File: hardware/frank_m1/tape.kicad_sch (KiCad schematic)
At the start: 11 parts, among them J11 SJ1-353XNG, Q1 BC850, Q2 BC850

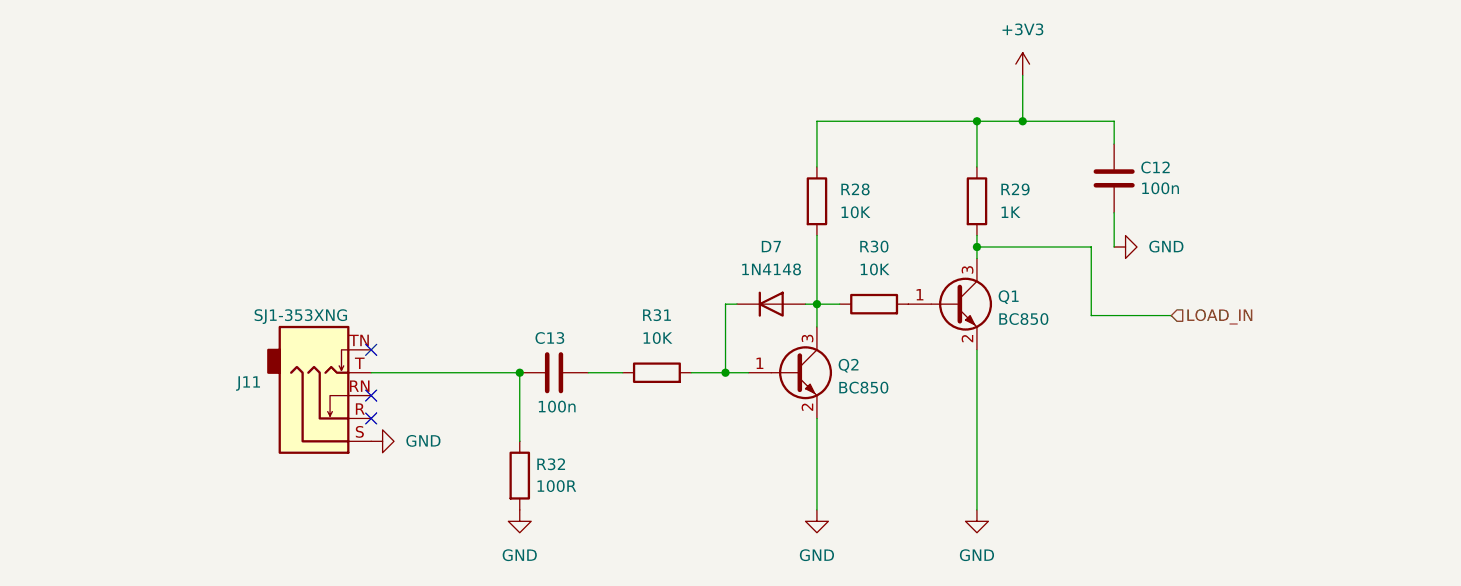
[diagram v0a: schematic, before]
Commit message: FRANK M1 2.03 & xt8086 WIP
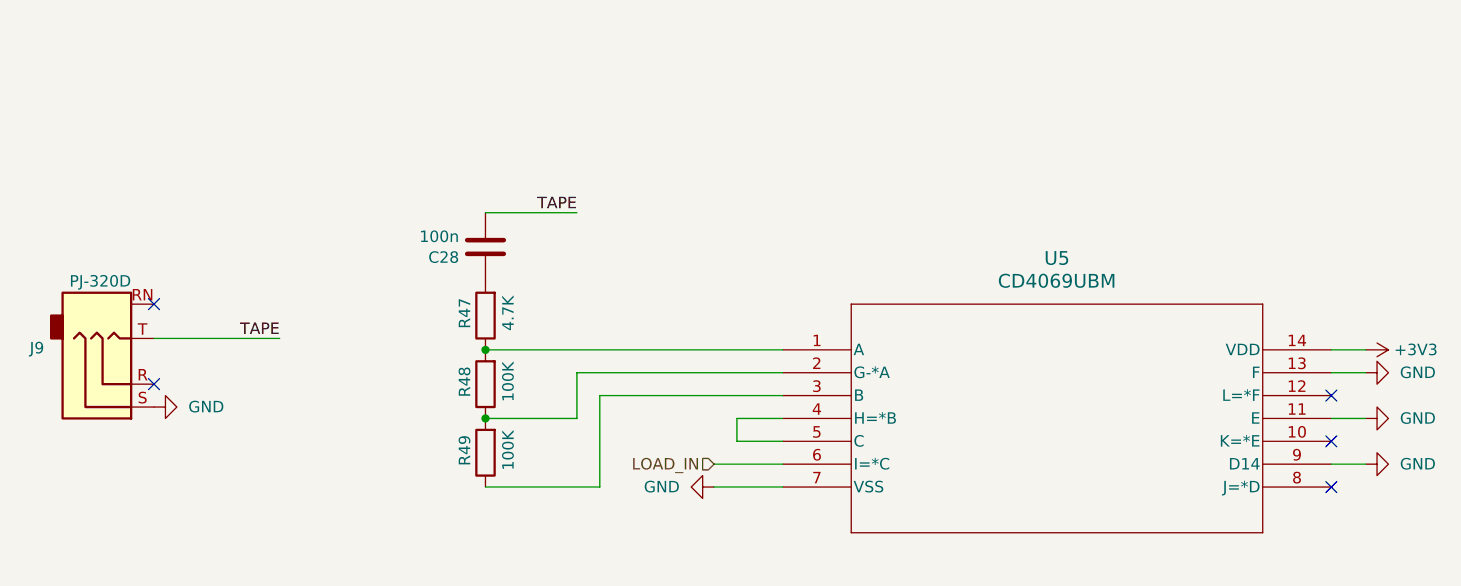
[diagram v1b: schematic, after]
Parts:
- removed C12, C13: 100n, FRANK:Capacitor (0805), symbol Device:C
- removed D7: 1N4148, FRANK:Diode (SOD-323), symbol Device:D
- removed Q1, Q2: BC850, FRANK:SOT-23, symbol Transistor_BJT:BC850
- removed R28, R30, R31: 10K, FRANK:Resistor (0805), symbol Device:R
- removed R29: 1K, FRANK:Resistor (0805), symbol Device:R
- removed R32: 100R, FRANK:Resistor (0805), symbol Device:R
- added C28: 100n, FRANK:C_0805_2012Metric, symbol Device:C
- added R47: 4.7K, FRANK:R_0805_2012Metric, symbol Device:R
- added R48, R49: 100K, FRANK:R_0805_2012Metric, symbol Device:R
- added U5: CD4069UBM, FRANK:SOIC127P600X175-14N, symbol FRANK:CD4069UBE
- J9: renamed from J11; value SJ1-353XNG -> PJ-320D; footprint FRANK:Jack (3.5mm) -> FRANK:Jack (3.5mm, PJ-320D); AliExpress https://www.aliexpress.com/item/1005006710837751.html -> https://www.aliexpress.com/item/4001158231104.html
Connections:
- net +3V3: now also U5.14 (VDD)
- net GND: now also U5.11 (E), U5.13 (F), U5.7 (VSS), U5.9 (D14)
- net LOAD_IN: now also U5.6 (I=*C)
- net TAPE: now reaches J9.T
- net TAPE: now also C28.2
- new net: R48.1, R49.2, U5.2 (G-*A)
- new net: R47.1, R48.2, U5.1 (A)
- new net: R49.1, U5.3 (B)
- new net: U5.4 (H=*B), U5.5 (C)
- new net: C28.1, R47.2
- no-connect marks 3 -> 5
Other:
- title: FRANK M1 -> ${NAME} ${MODEL}
